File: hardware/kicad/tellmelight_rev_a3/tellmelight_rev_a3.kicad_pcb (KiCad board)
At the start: 4 copper layers, 76 x 56 mm, 60 parts, among them J1 USB_C, SW1 BOOT, SW2 RESET, U1 RP2040, U2 LP5024, U3 W25Q32JVSS, U4 AP2112K-3.3, U5 TPD2EUSB30, U6 TPD1E05U06DPY, Y1 12MHz

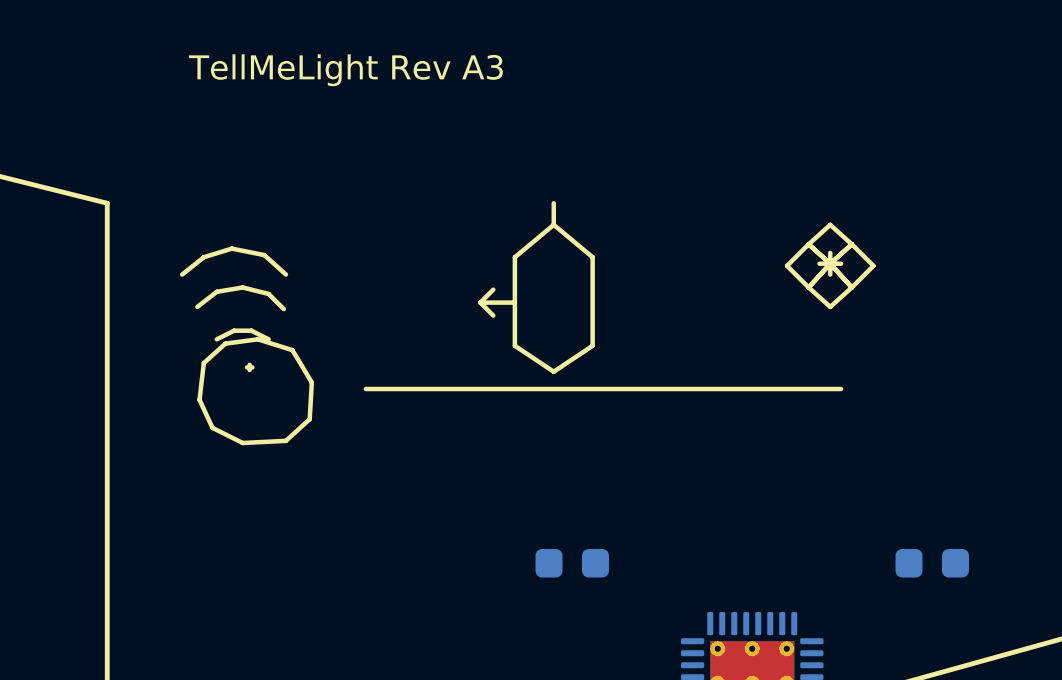
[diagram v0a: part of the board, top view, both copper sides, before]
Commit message: design: refine rev a3 avatar watermark
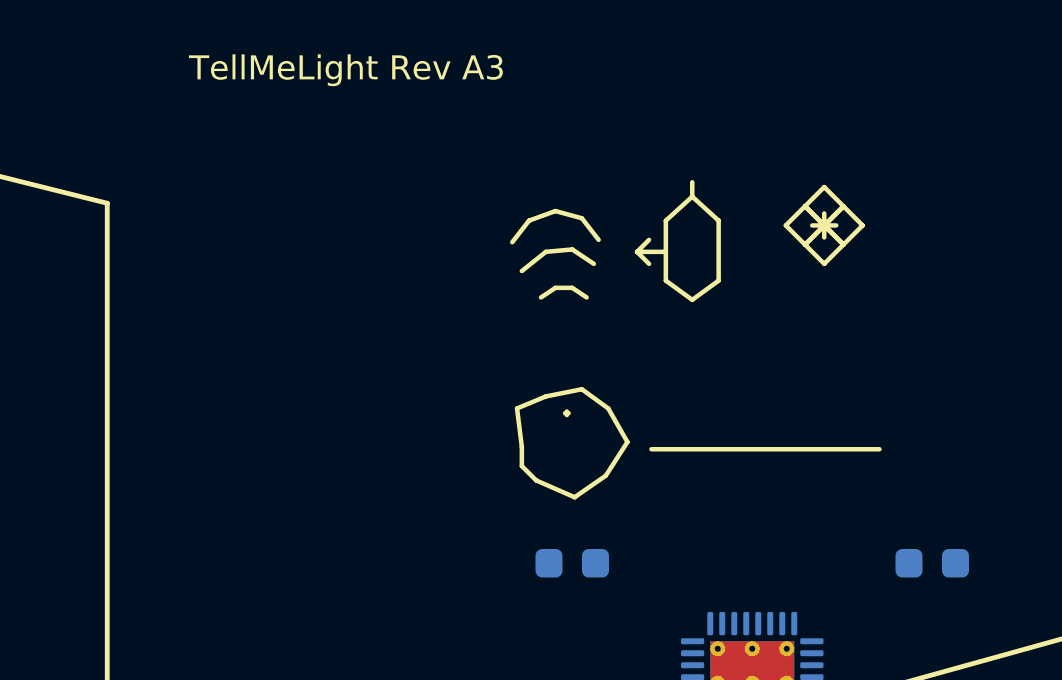
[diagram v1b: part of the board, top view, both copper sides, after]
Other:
- board text added: "Avatar watermark A1 separated"
